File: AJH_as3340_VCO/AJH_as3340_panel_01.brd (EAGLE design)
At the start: 30 x 128.5 mm, 1 part

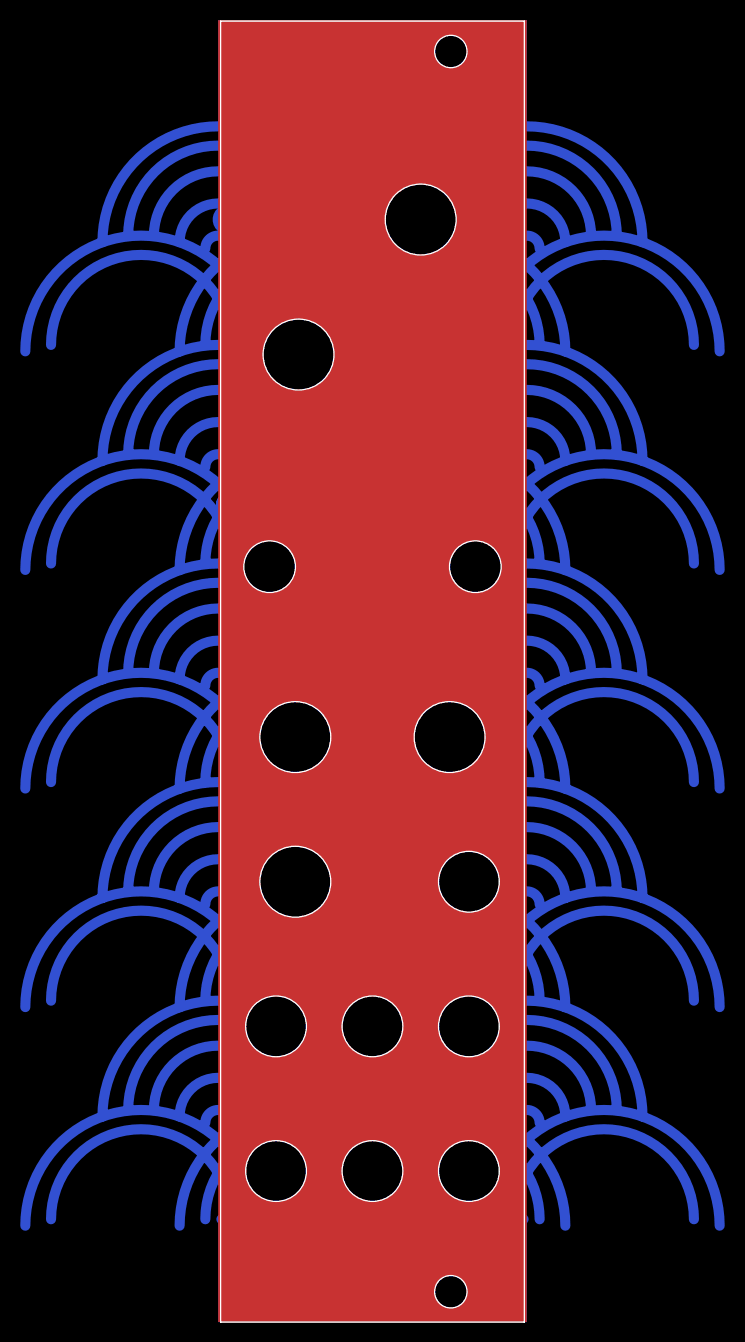
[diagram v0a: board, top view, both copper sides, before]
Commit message: Refined Panel Design
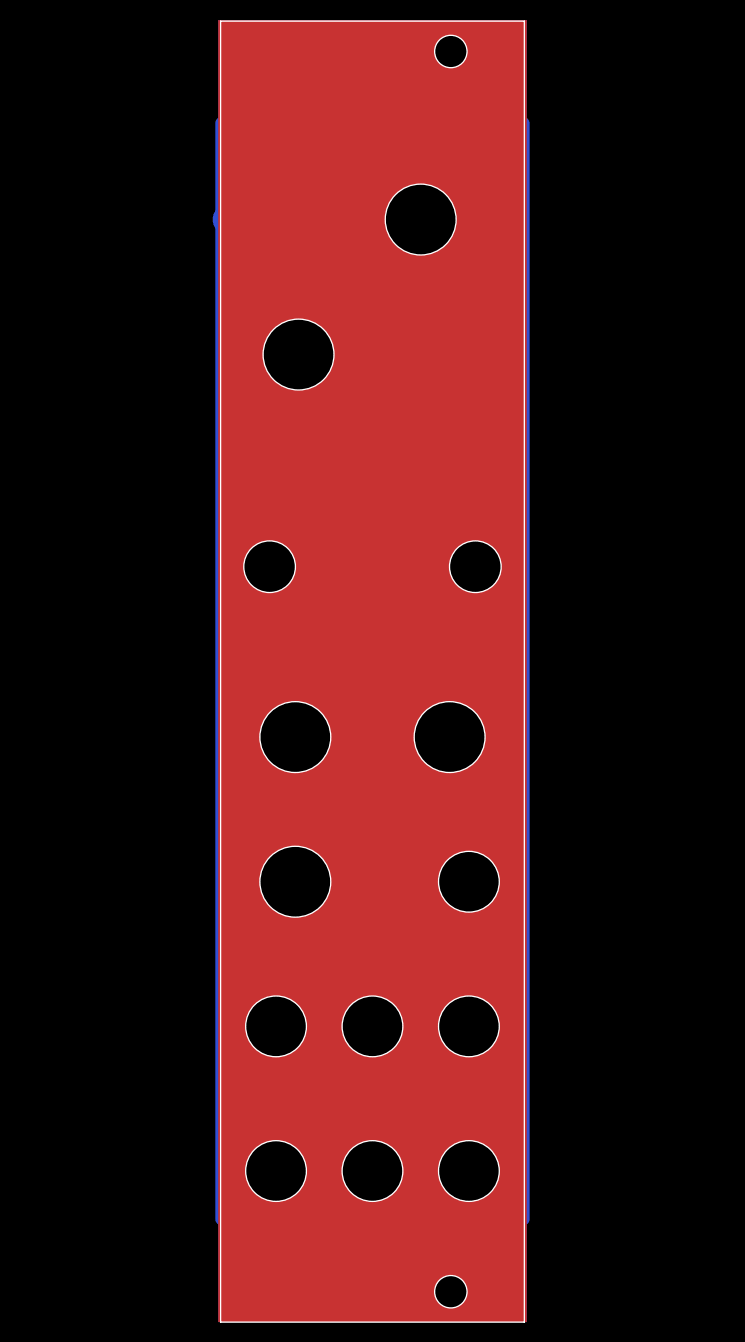
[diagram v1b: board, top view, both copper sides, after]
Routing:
- net GND: track 0.00 -> 232.2 mm
- net S$56: track 22.9 -> 8.40 mm
- net S$28: track 22.9 -> 8.40 mm
- net S$23: track 22.9 -> 8.40 mm
- net S$125: track 22.9 -> 8.40 mm
- net S$119: track 22.9 -> 8.40 mm
- net S$8: track 22.9 -> 8.40 mm
- net S$42: track 22.9 -> 8.40 mm
- net S$4: track 22.9 -> 8.40 mm
- net S$48: track 22.9 -> 8.40 mm
- net S$131: track 22.9 -> 8.40 mm
- net S$9: track 17.8 -> 3.55 mm
- net S$29: track 17.8 -> 3.55 mm
- net S$47: track 17.8 -> 3.55 mm
- net S$43: track 17.8 -> 3.55 mm
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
